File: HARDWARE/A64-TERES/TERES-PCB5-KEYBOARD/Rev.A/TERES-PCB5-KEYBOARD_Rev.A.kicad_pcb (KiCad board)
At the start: 2 copper layers, 68.5 x 34.5 mm, 78 parts, among them P1 CONN_01X24, P2 CONN_01X06, P3 CONN_01X12, U1 ATMEGA16U4-A, Y1 16.000MHz/SMD5x3.2/12pF

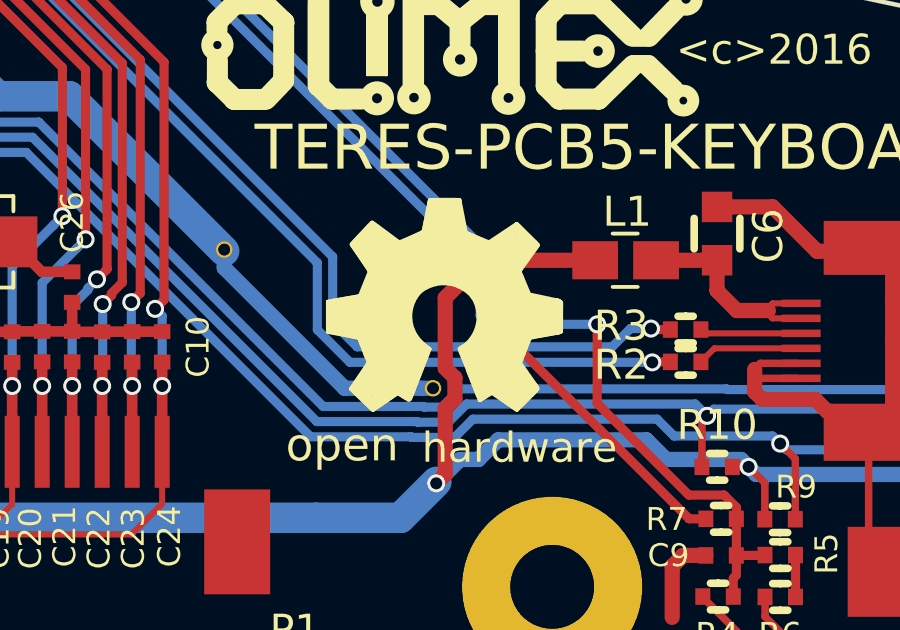
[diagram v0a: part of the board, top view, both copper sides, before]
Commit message: Update projects using KiCAD 6.0.7
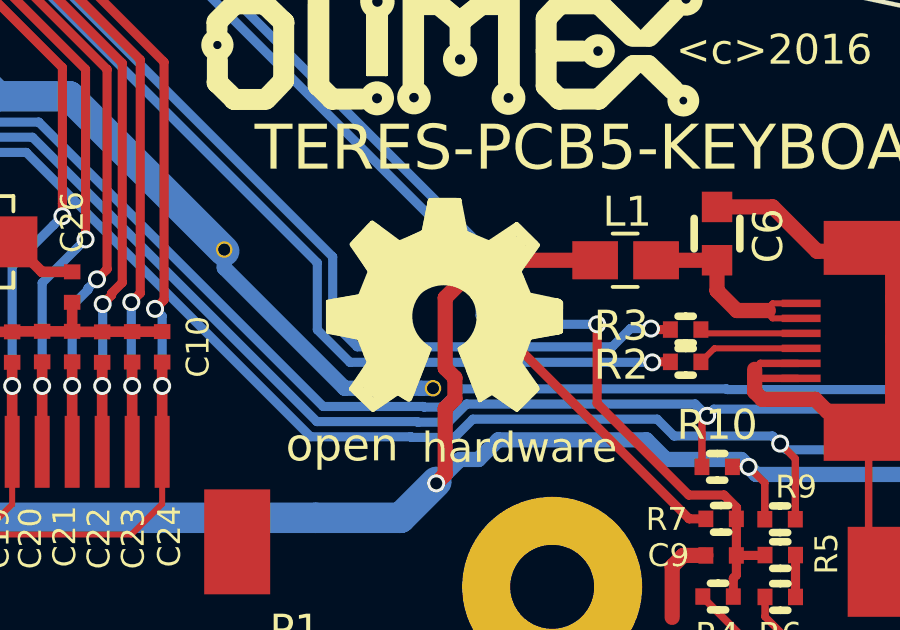
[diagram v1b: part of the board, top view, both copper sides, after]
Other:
- net class Default removed
